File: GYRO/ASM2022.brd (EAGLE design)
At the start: 22.5 x 21.3 mm, 27 parts, among them J1 47346-0001, J2 DF12-32-DS, J3 47346-0001, J4 DF12-32-DP, Q1 DMP2035U, U2 FT231XQ-R

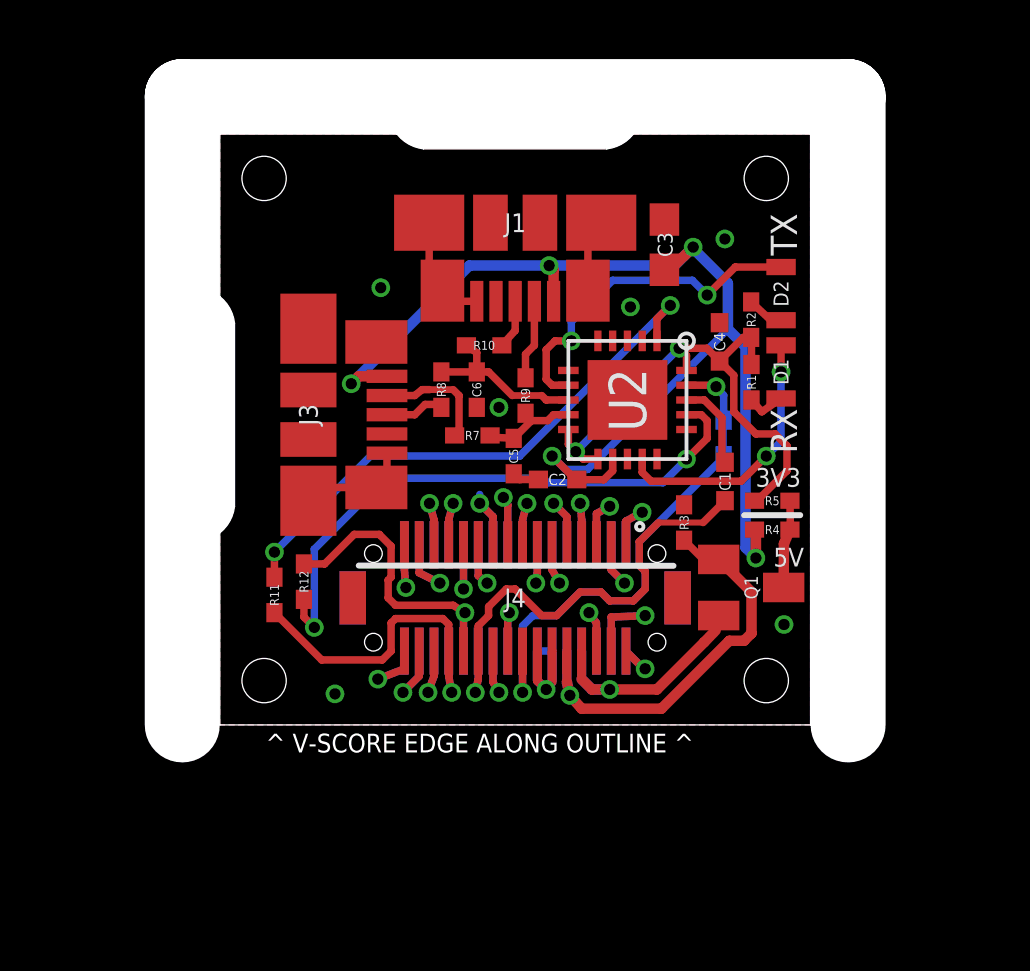
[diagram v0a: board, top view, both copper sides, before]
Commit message: asdsa
asd
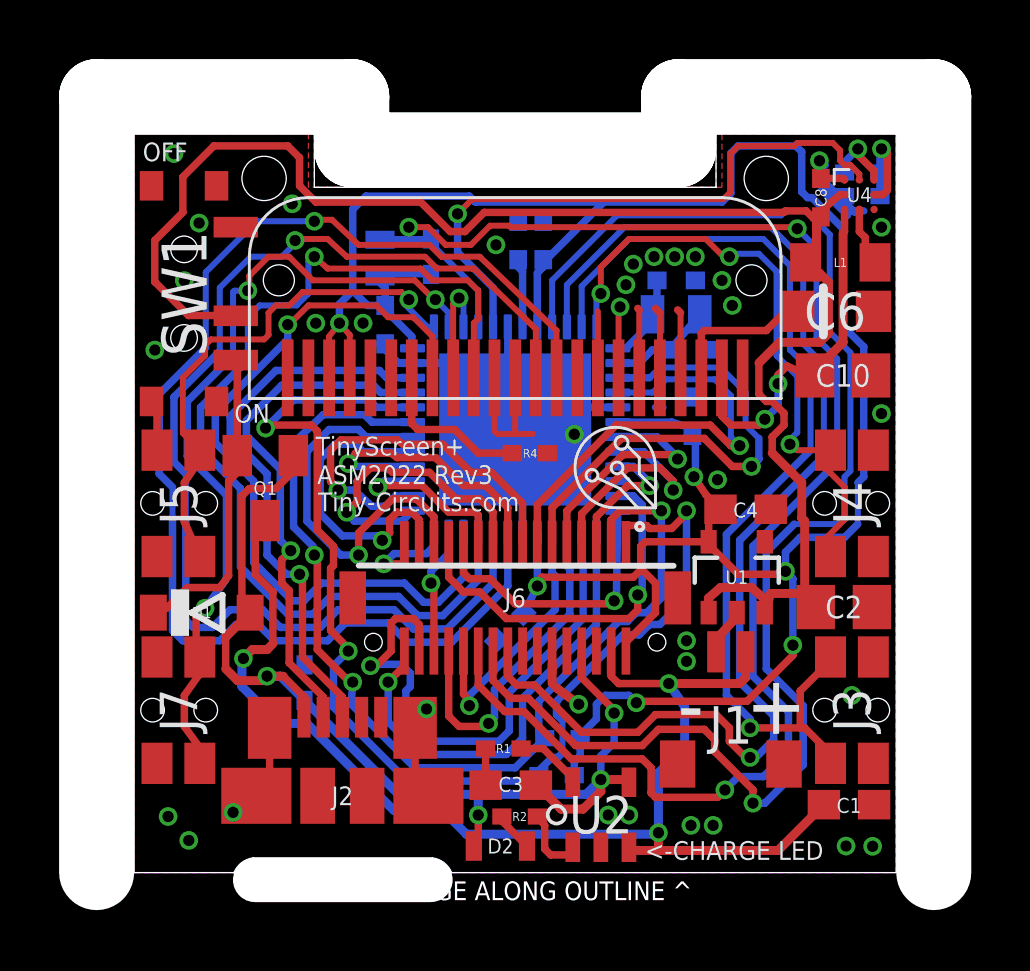
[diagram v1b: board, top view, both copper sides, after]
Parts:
- removed R10: 27.0, tinycircuits:0402
- removed R11, R12: 1.00K, tinycircuits:0402
- added C10: 10uF, tinycircuits:C0805
- added C11, C12, C13, C14, C9: .1uF, tinycircuits:C0402
- added C7: 22pF, tinycircuits:C0402
- added C8: 4.7uF, tinycircuits:C0402
- added D3: CD0603, tinycircuits:0603
- added J5, J7: EVP-ANDA1A, tinycircuits:PTS840GKP
- added J6: DF12-32-DP, tinycircuits:DF12-32-DP
- added L1: 22uH, tinycircuits:R0805
- added SW1: PCM12SMTR, tinycircuits:PCM12SMTR
- added U1: XC6210B33, tinycircuits:SOT-25
- added U3: UG-9664HDDAG01, tinycircuits:OLED_DISPLAY
- added U4: FAN5340, tinycircuits:WLCSP8_1_57X1_57
- added U5: ATSAMD21G18A, tinycircuits:QFN48
- added Y1: 32.7680, tinycircuits:ABS06
- C1: value 0.1uF -> 4.7uF; device tinycircuits:C0402 -> tinycircuits:C0603
- C2: value 0.1uF -> 10uF; device tinycircuits:C0402 -> tinycircuits:C0805
- C4: value 0.1uF -> 10uF; device tinycircuits:C0402 -> tinycircuits:C0603
- C5: value 47pF -> 22pF; device tinycircuits:0402 -> tinycircuits:C0402
- C6: value 47pF -> 4.7uF; device tinycircuits:0402 -> tinycircuits:1206_CAP_TANT
- D1: value AMBER -> MBR120; device tinycircuits:LNJ_LED -> tinycircuits:SOD-123FL
- J1: value 47346-0001 -> SM02B-SRSS-TB(LF)(SN); device tinycircuits:MICRO_USB -> tinycircuits:JST_SH_2X1
- J2: value DF12-32-DS -> 47346-0001; device tinycircuits:DF12-32-DS -> tinycircuits:MICRO_USB
- J3: value 47346-0001 -> EVP-ANDA1A; device tinycircuits:MICRO_USB -> tinycircuits:PTS840GKP
- J4: value DF12-32-DP -> EVP-ANDA1A; device tinycircuits:DF12-32-DP -> tinycircuits:PTS840GKP
- R1: value 1.00K -> 5K
- R2: value 1.00K -> 1k
- R3: value 1.00K -> 100k
- R4: value 0.0 -> 1.2M
- R5: value 0.0 -> 115k
- R6: value 0.0 -> 4.7k; device tinycircuits:0402_SHORT -> tinycircuits:0402
- R7, R8, R9: value 27.0 -> 10K
- U2: value FT231XQ-R -> MCP73831; device tinycircuits:QFN20 -> tinycircuits:SOT-23
- moved D1 21.2 mm to (9.39, 13.8), turned to 0 degrees
- moved D2 21.0 mm to (19.5, 5.90), turned to 90 degrees
- moved J3 20.9 mm to (31.4, 10.5), turned to 90 degrees
- moved C3 19.0 mm to (19.9, 7.96), turned to 180 degrees
- moved R2 18.6 mm to (20.1, 6.90), turned to 0 degrees
- moved J1 18.5 mm to (27.3, 10.0), turned to 0 degrees
- moved Q1 16.8 mm to (11.5, 18.0), turned to 180 degrees
- moved R1 15.0 mm to (19.6, 9.20), turned to 180 degrees
- moved U2 14.1 mm to (22.9, 6.96), turned to 0 degrees
- moved R3 13.9 mm to (12.9, 11.4), flipped to the bottom
- moved R8 12.5 mm to (21.6, 9.55), flipped to the bottom, turned to 180 degrees
- moved C6 12.4 mm to (30.8, 24.0), turned to 0 degrees
- moved R7 11.8 mm to (21.4, 8.30), flipped to the bottom, turned to 180 degrees
- moved J4 11.8 mm to (31.4, 17.5), turned to 90 degrees
- moved C1 11.7 mm to (31.3, 7.30), turned to 0 degrees
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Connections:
- removed net 3V3OUT: C4.1, R1.2, R2.2, R5.1, U2.10, U2.11, U2.20
- removed net DTR: C1.1, U2.18
- removed net N$10: R12.2, U2.17
- removed net N$16: D1.C, U2.14
- removed net N$4: Q1.C, R4.2, R5.2
- removed net RSV0: J2.20, J4.20
- removed net RSV1: J2.18, J4.18
- removed net RTS: R6.1, U2.19
- removed net USBDM: C5.1, R7.2, R9.2, U2.9
- removed net USBDP: C6.1, R10.2, R8.2, U2.8
- removed net USBVCC: C2.1, C3.1, J1.1, J3.1, R4.1, U2.12
- new net +12V: C10.1, U3.22, U4.C1
- new net AD4: U5.10
- new net AD5: J3.1, J3.2, U5.47
- new net ATN/IO38: U3.8, U5.22
- new net DBG_RXD: J7.1, J7.2, U5.38
- new net DBG_TXD: J5.1, J5.2, U5.37
- new net MISO_ALT: U3.10, U5.21
- new net MOSI_ALT: U3.14, U5.19
- new net N$11: R4.2, U3.7
- new net N$12: C6.1, U3.21
- new net N$13: R5.1, U4.A3
- new net N$15: U3.15
- new net RX_LED/IO25/AIN11: J4.1, J4.2, U5.48
- new net SCK_ALT: U3.13, U5.20
- new net SWCLK: J6.20, U5.45
- new net SWDIO: J6.18, U5.46
- new net TX_LED/IO26: U3.9, U5.39
- new net USB_HOST_EN/IO27: U4.A2, U5.41
- new net USB_N: J2.2, U5.33
- new net USB_P: J2.3, U5.34
- new net VCC_IN: C2.1, C8.1, L1.1, SW1.2, U1.1, U1.3, U4.B1
- new net V_FB: R5.2, R6.2, U4.B3
- net +3V3: now also J6.6; no longer J2.6, J4.6
- net +5V: now also C3.1, D1.A, D2.A, J2.1, J6.8, Q1.B, R3.2, U2.4; no longer J2.8, J4.8, Q1.E
- net AD0: now also J6.11, U5.3; no longer J2.11, J4.11
- net AD1: now also J6.9, U5.7; no longer J2.9, J4.9
- net AD2: now also J6.7, U5.8; no longer J2.7, J4.7
- net AD3: now also J6.5, U5.9; no longer J2.5, J4.5
- net AD4/SDA: now also J6.3, R8.1, U5.31; no longer J2.3, J4.3
- net AD5/SCL: now also J6.1, R7.1, U5.32; no longer J2.1, J4.1
- net AREF: now also J6.13, U5.4; no longer J2.13, J4.13
- net GND: now also C1.2, C10.2, C11.2, C12.2, C13.2, C14.2, C7.2, C8.2, C9.2, J1.1, J2.5, J2.P1, J2.P2, J2.P3, J2.P4, J2.P5, J2.P6, J3.3, J3.4, J4.3, J4.4, J5.3, J5.4, J6.12, J6.14, J7.3, J7.4, R1.2, R4.1, R6.1, SW1.W1, SW1.W2, SW1.W3, SW1.W4, U1.2, U2.2, U3.11, U3.12, U3.16, U3.17, U3.18, U3.19, U3.2, U3.20, U3.5, U3.6, U4.A1, U4.C3, U5.18, U5.35, U5.42, U5.5, U5.EXP; no longer J1.5, J1.P1, J1.P2, J1.P3, J1.P4, J1.P5, J1.P6, J2.12, J2.14, J3.5, J3.P1, J3.P2, J3.P3, J3.P4, J3.P5, J3.P6, J4.12, J4.14, U2.13, U2.21, U2.3
- net IO0: now also J6.24, U5.16; no longer J2.24, J4.24, R12.1
- net IO1: now also J6.26, U5.15; no longer J2.26, J4.26, R11.1
- net IO2: now also J6.28, U5.23; no longer J2.28, J4.28
- net IO3: now also J6.30, U5.14; no longer J2.30, J4.30
- net IO4: now also J6.32, U5.13; no longer J2.32, J4.32
- net IO5: now also J6.31, U5.24; no longer J2.31, J4.31
- net IO6: now also J6.29, U5.29; no longer J2.29, J4.29
- net IO7: now also J6.27, U5.30; no longer J2.27, J4.27
- net IO8: now also J6.25, U5.11; no longer J2.25, J4.25
- net IO9: now also J6.23, U5.12; no longer J2.23, J4.23
- net MISO: now also J6.17, U5.28; no longer J2.17, J4.17
- net MOSI: now also J6.19, U5.25; no longer J2.19, J4.19
- net N$1: now also C5.1, U5.1, Y1.1; no longer J3.2, R7.1
- net N$2: now also D1.C, Q1.E, SW1.3; no longer J1.2, R9.1
- net N$3: now also C7.1, U5.2, Y1.2; no longer J1.3, R10.1
- net N$5: now also R2.1; no longer U2.7
- net N$6: now also U2.5; no longer D1.A
- net N$7: now also R2.2, U2.1; no longer D2.A, R2.1
- net N$8: now also C9.1, U5.43; no longer J3.3, R8.1
- net N$9: now also L1.2, U4.C2; no longer R11.2, U2.1
- net RESET: now also D3.A, J6.22, R9.1, U5.40; no longer C1.2, J2.22, J4.22
- net RSV2: now also J6.16; no longer J2.16, J4.16, R6.2
- net SCK: now also J6.15, U5.26; no longer J2.15, J4.15
- net SS: now also J6.21, U5.27; no longer J2.21, J4.21
- net VBATT: now also C1.1, J1.2, J6.4, Q1.C, U2.3; no longer J2.4, J4.4
- net VCC: now also C11.1, C12.1, C13.1, C14.1, C4.1, D3.C, J6.2, R7.2, R8.2, R9.2, U1.5, U3.3, U3.4, U5.17, U5.36, U5.44, U5.6; no longer J2.2, J4.2
- net VIN: now also J6.10; no longer J2.10, J4.10, Q1.B, R3.2
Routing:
- net VCC: track 1.80 -> 91.3 mm, vias 1 -> 6
- net VCC_IN: track 0.00 -> 54.6 mm
- net SWCLK: track 0.00 -> 47.8 mm, vias 0 -> 1
- net MOSI_ALT: track 0.00 -> 43.8 mm, vias 0 -> 1
- net USBVCC: track 40.9 -> 0.00 mm, vias 5 -> 0
- net SWDIO: track 0.00 -> 40.9 mm, vias 0 -> 1
- net SCK_ALT: track 0.00 -> 40.3 mm, vias 0 -> 1
- net VBATT: track 4.60 -> 42.9 mm, vias 1 -> 3
- net RESET: track 16.2 -> 54.4 mm, vias 1 -> 3
- net AD5/SCL: track 2.85 -> 40.3 mm, vias 1 -> 3
- net GND: track 16.5 -> 53.2 mm, vias 7 -> 35
- net MISO_ALT: track 0.00 -> 33.8 mm, vias 0 -> 1
- net AD5: track 0.00 -> 33.1 mm, vias 0 -> 1
- net AD4/SDA: track 2.97 -> 35.0 mm, vias 1 -> 3
- net +5V: track 9.02 -> 37.0 mm, vias 1 -> 4
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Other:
- board size 22.5 x 21.3 mm -> 28.3 x 26.5 mm
- board text added: "+"
- board text added: "-"
- board text added: "3"
- board text added: "<-CHARGE LED"
- board text added: "AS-PCB-ASM2022"
- board text added: "ASM2022 Rev3"
- board text added: "OFF"
- board text added: "ON"
- board text added: "TinyScreen+"
- board text removed: "3V3"
- board text removed: "5V"
- board text removed: "6"
- board text removed: "AS-PCB-ASD2101"
- board text removed: "ASD2101 - Rev6"
- board text removed: "R6"
- board text removed: "RX"
- board text removed: "TX"
- board text removed: "TinyShield - USB & ICP"
- board text removed: "USB TinyShield"
